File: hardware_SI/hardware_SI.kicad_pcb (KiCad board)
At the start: 2 copper layers, 228 x 147.6 mm, 58 parts, among them J1 Barrel_Jack_Switch, J2 Conn_01x07_Female, J3 USB_B_Micro, Q1 SI2323DS-T1, Q2 SI2323DS-T1, SW1 SW_SPDT, U1 OMEGA2+, U2 LTC4085EDEPBF, U3 TPS61200DRC, U4 LD1117S33TR_SOT223, U5 MAX6369, U6 MCP3021, U7 USBLC6-2SC6, U8 CH340N

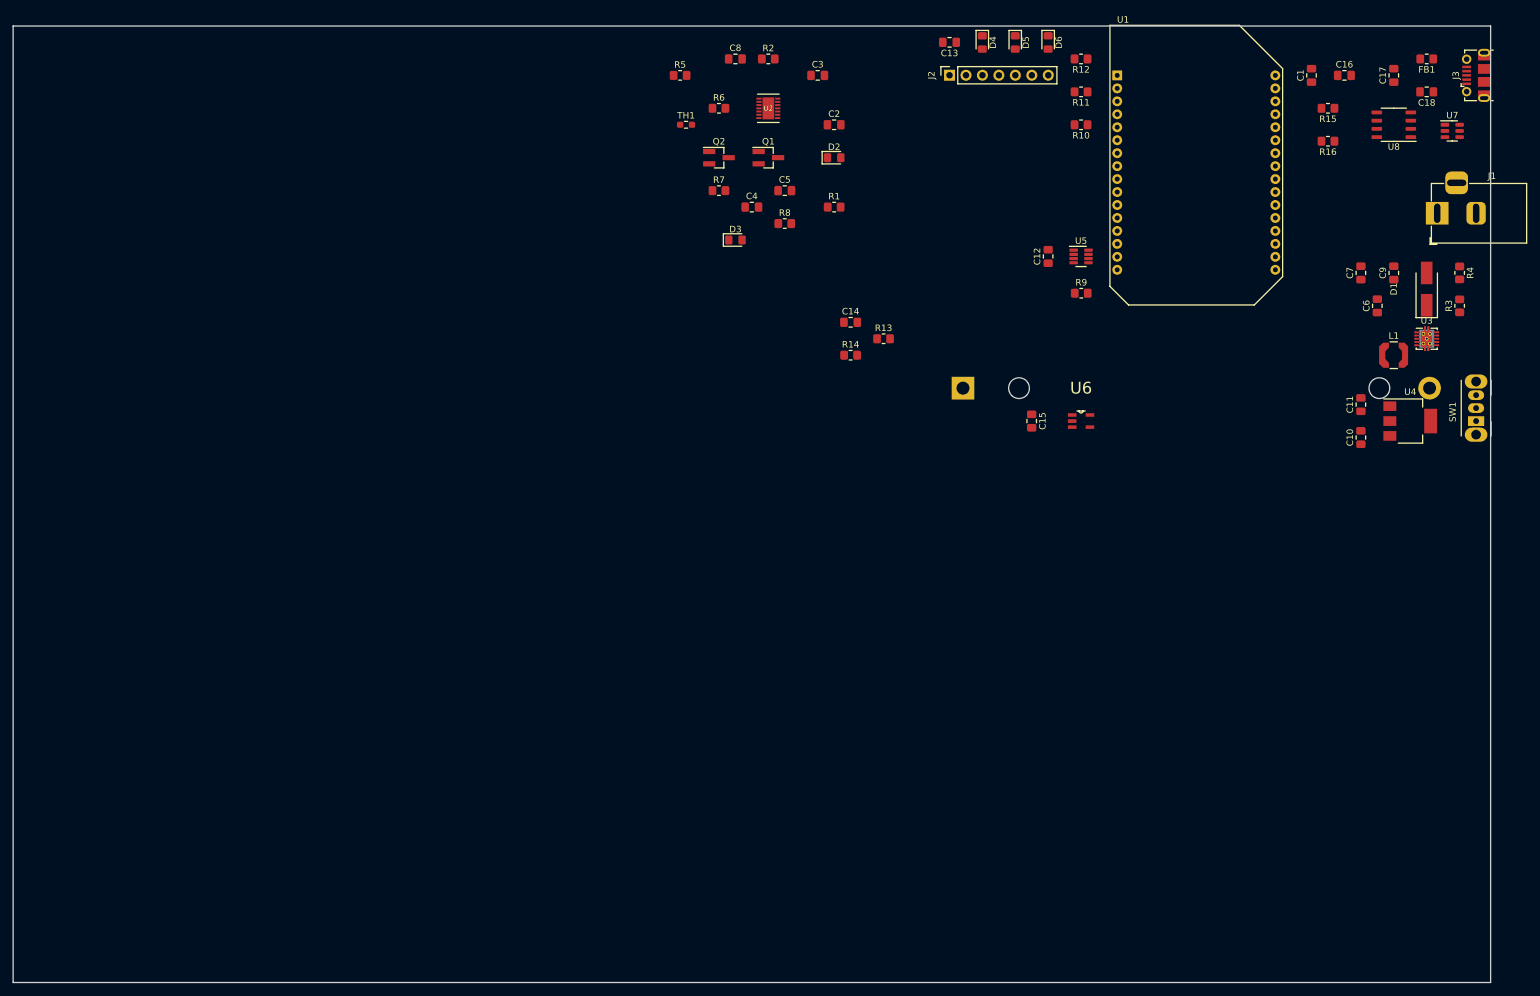
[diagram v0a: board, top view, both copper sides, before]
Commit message: PCB V2
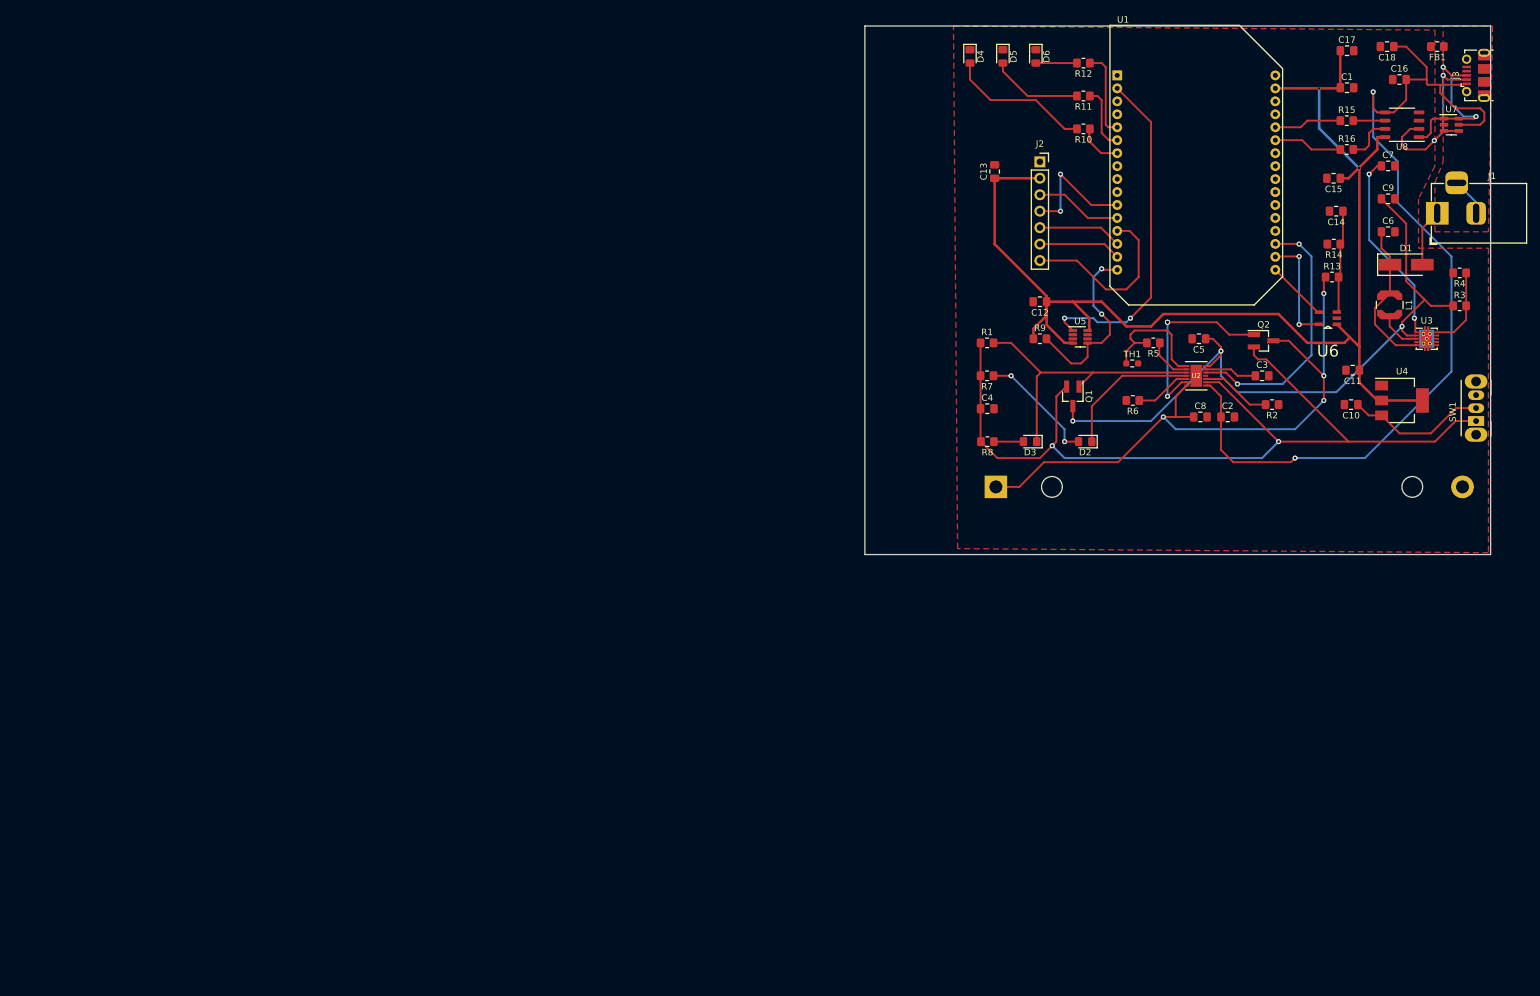
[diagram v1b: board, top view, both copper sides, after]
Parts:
- moved R2 94.3 mm to (217.4, 81.3), turned to 180 degrees
- moved C8 90.6 mm to (206.4, 83.2)
- moved Q2 88.7 mm to (216.1, 71.4)
- moved R5 83.9 mm to (199.1, 71.8), turned to 180 degrees
- moved C3 82.8 mm to (215.9, 76.8)
- moved R6 78.2 mm to (195.9, 80.6), turned to 180 degrees
- moved TH1 78.1 mm to (195.9, 74.9)
- moved U2 77.9 mm to (205.7, 76.8), turned to 180 degrees
- moved C14 76.9 mm to (227.3, 51.4), turned to 180 degrees
- moved R14 76.5 mm to (227.0, 56.5), turned to 180 degrees
- moved C2 75.6 mm to (210.6, 83.2)
- moved R13 69.9 mm to (226.7, 61.6)
- moved C5 67.9 mm to (206.1, 71.1), turned to 180 degrees
- moved C15 59.8 mm to (226.9, 46.4), turned to 180 degrees
- moved Q1 59.7 mm to (186.7, 80.0), turned to -90 degrees
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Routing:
- net +3V3: track 0.00 -> 190.8 mm, vias 0 -> 2
- net +5VA: track 0.00 -> 144.9 mm
- net +5VL: track 0.00 -> 143.2 mm, vias 0 -> 2
- net +5VP: track 0.00 -> 105.6 mm, vias 0 -> 2
- net +BATT: track 0.00 -> 97.3 mm, vias 0 -> 3
- net /WDI: track 0.00 -> 52.1 mm, vias 0 -> 1
- net /sistema_alimentacion/*ACPR: track 0.00 -> 45.7 mm
- net /IO19: track 0.00 -> 40.5 mm
- net Net-(C7-Pad1): track 0.00 -> 29.8 mm
- net Net-(Q2-Pad1): track 0.00 -> 29.5 mm, vias 0 -> 3
- net Net-(J3-Pad2): track 0.00 -> 29.1 mm, vias 0 -> 1
- net /RST_W: track 0.00 -> 28.7 mm
- net /CS1: track 0.00 -> 27.5 mm
- net Net-(J3-Pad3): track 0.00 -> 26.2 mm
- net Net-(C6-Pad1): track 0.00 -> 23.6 mm
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- added copper zone on F.Cu, net GND
- added copper zone on F.Cu, net GNDPWR
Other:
- board size 228 x 147.6 mm -> 96.6 x 81.6 mm
